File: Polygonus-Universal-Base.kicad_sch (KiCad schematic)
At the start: 5 parts, among them J4 Polygonus_Plugs, J5 Conn_02x04_Top_Bottom, U1 WBO-Single-Module

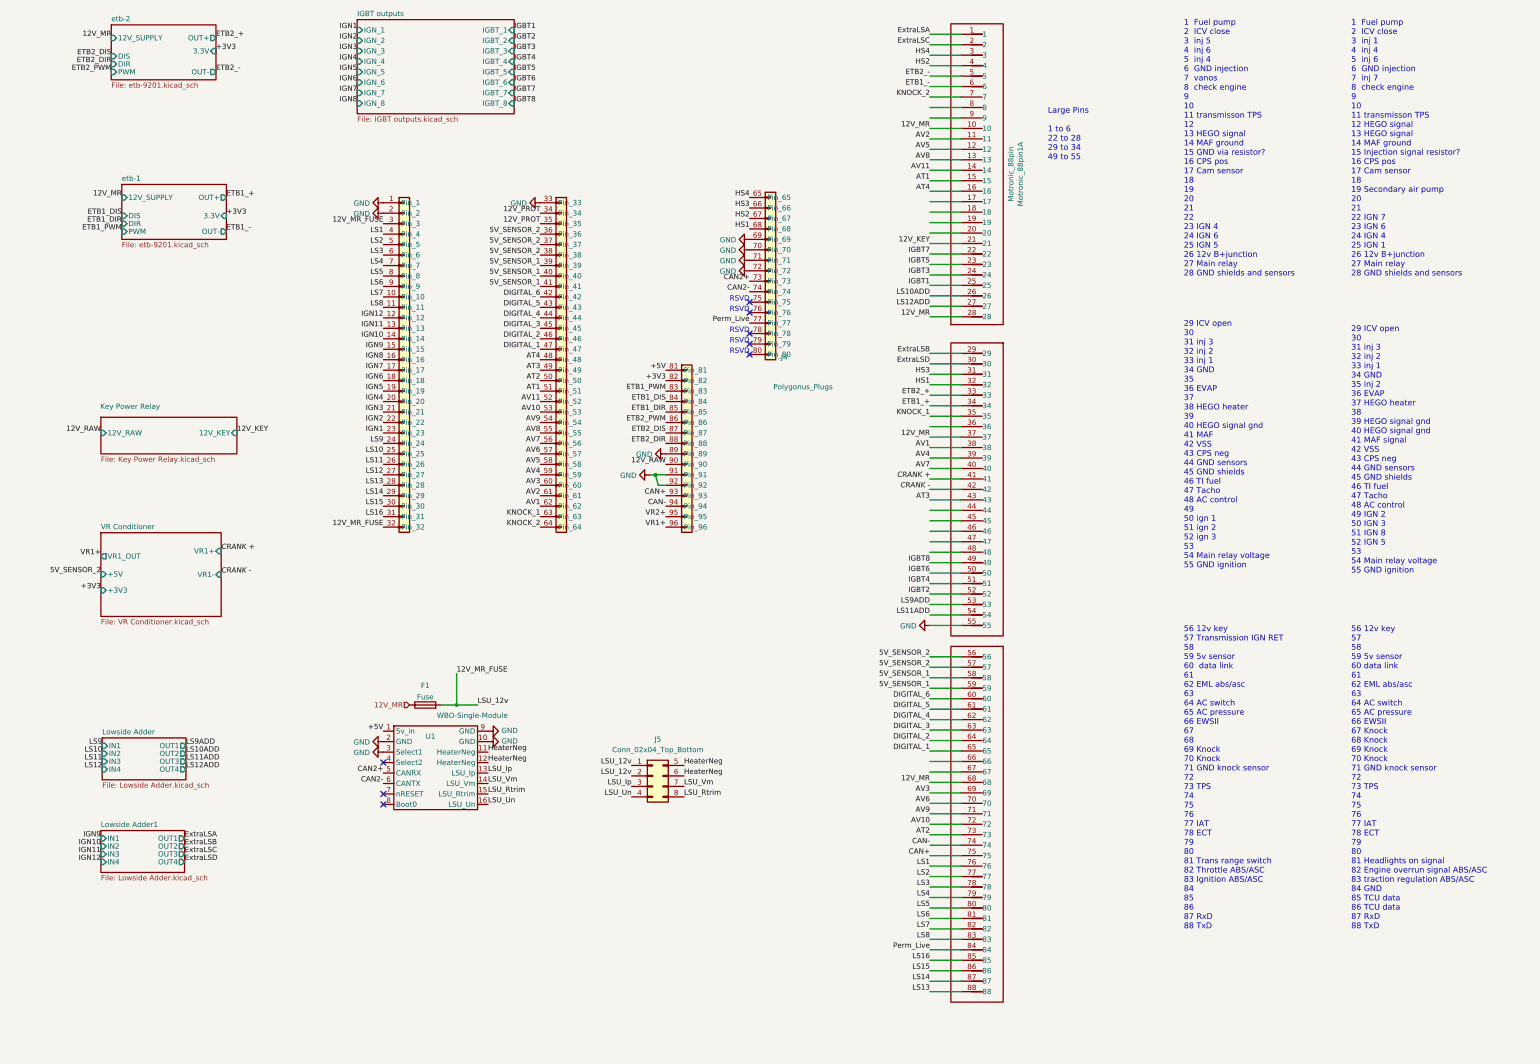
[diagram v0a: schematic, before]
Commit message: Competed board
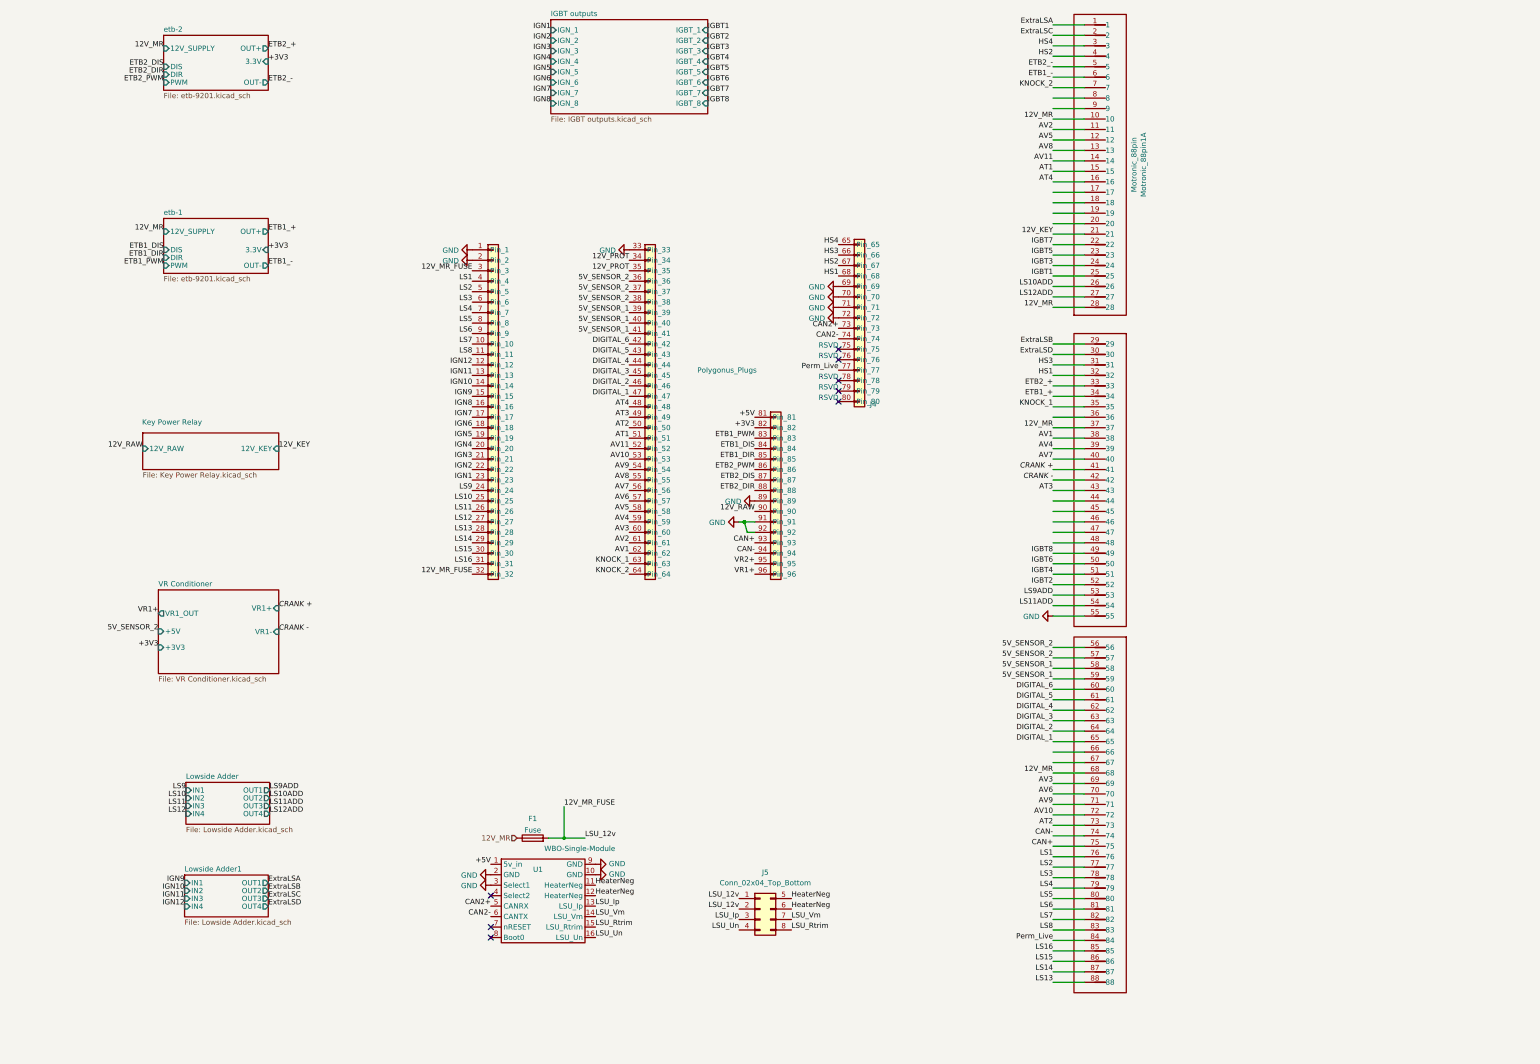
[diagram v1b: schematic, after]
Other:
- note removed: "1 Fuel pump 2 ICV close 3 inj 1 4 inj 4 5 inj 6 6 GND injection 7 inj 7 8 check engine 9 10 11 transmisson TPS 12 HEGO signal 13 HEGO signal 14 MAF ground 15 Injection signal resistor? 16 CPS pos 17 Cam sensor 18 19 Secondary air pump 20 21 22 IGN 7 23 IGN 6 24 IGN 4 25 IGN 1 26 12v B+junction 27 Main relay 28 GND shields and sensors"
- note removed: "1 Fuel pump 2 ICV close 3 inj 5 4 inj 6 5 inj 4 6 GND injection 7 vanos 8 check engine 9 10 11 transmisson TPS 12 13 HEGO signal 14 MAF ground 15 GND via resistor? 16 CPS pos 17 Cam sensor 18 19 20 21 22 23 IGN 4 24 IGN 6 25 IGN 5 26 12v B+junction 27 Main relay 28 GND shields and sensors"
- note removed: "29 ICV open 30 31 inj 3 32 inj 2 33 inj 1 34 GND 35 36 EVAP 37 38 HEGO heater 39 40 HEGO signal gnd 41 MAF 42 VSS 43 CPS neg 44 GND sensors 45 GND shields 46 TI fuel 47 Tacho 48 AC control 49 50 ign 1 51 ign 2 52 ign 3 53 54 Main relay voltage 55 GND ignition"
- note removed: "29 ICV open 30 31 inj 3 32 inj 2 33 inj 1 34 GND 35 inj 2 36 EVAP 37 HEGO heater 38 39 HEGO signal gnd 40 HEGO signal gnd 41 MAF signal 42 VSS 43 CPS neg 44 GND sensors 45 GND shields 46 TI fuel 47 Tacho 48 AC control 49 IGN 2 50 IGN 3 51 IGN 8 52 IGN 5 53 54 Main relay voltage 55 GND ignition"
- note removed: "56 12v key 57 58 59 5v sensor 60 data link 61 62 EML abs/asc 63 64 AC switch 65 AC pressure 66 EWSII 67 Knock 68 Knock 69 Knock 70 Knock 71 GND knock sensor 72 73 TPS 74 75 76 77 IAT 78 ECT 79 80 81 Headlights on signal 82 Engine overrun signal ABS/ASC 83 traction regulation ABS/ASC 84 GND 85 TCU data 86 TCU data 87 RxD 88 TxD"
- note removed: "56 12v key 57 Transmission IGN RET 58 59 5v sensor 60 data link 61 62 EML abs/asc 63 64 AC switch 65 AC pressure 66 EWSII 67 68 69 Knock 70 Knock 71 GND knock sensor 72 73 TPS 74 75 76 77 IAT 78 ECT 79 80 81 Trans range switch 82 Throttle ABS/ASC 83 Ignition ABS/ASC 84 85 86 87 RxD 88 TxD"
- note removed: "Large Pins 1 to 6 22 to 28 29 to 34 49 to 55"
- moved on the sheet: F1, J4, J5, Motronic_88pin1A, U1

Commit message: upgraded
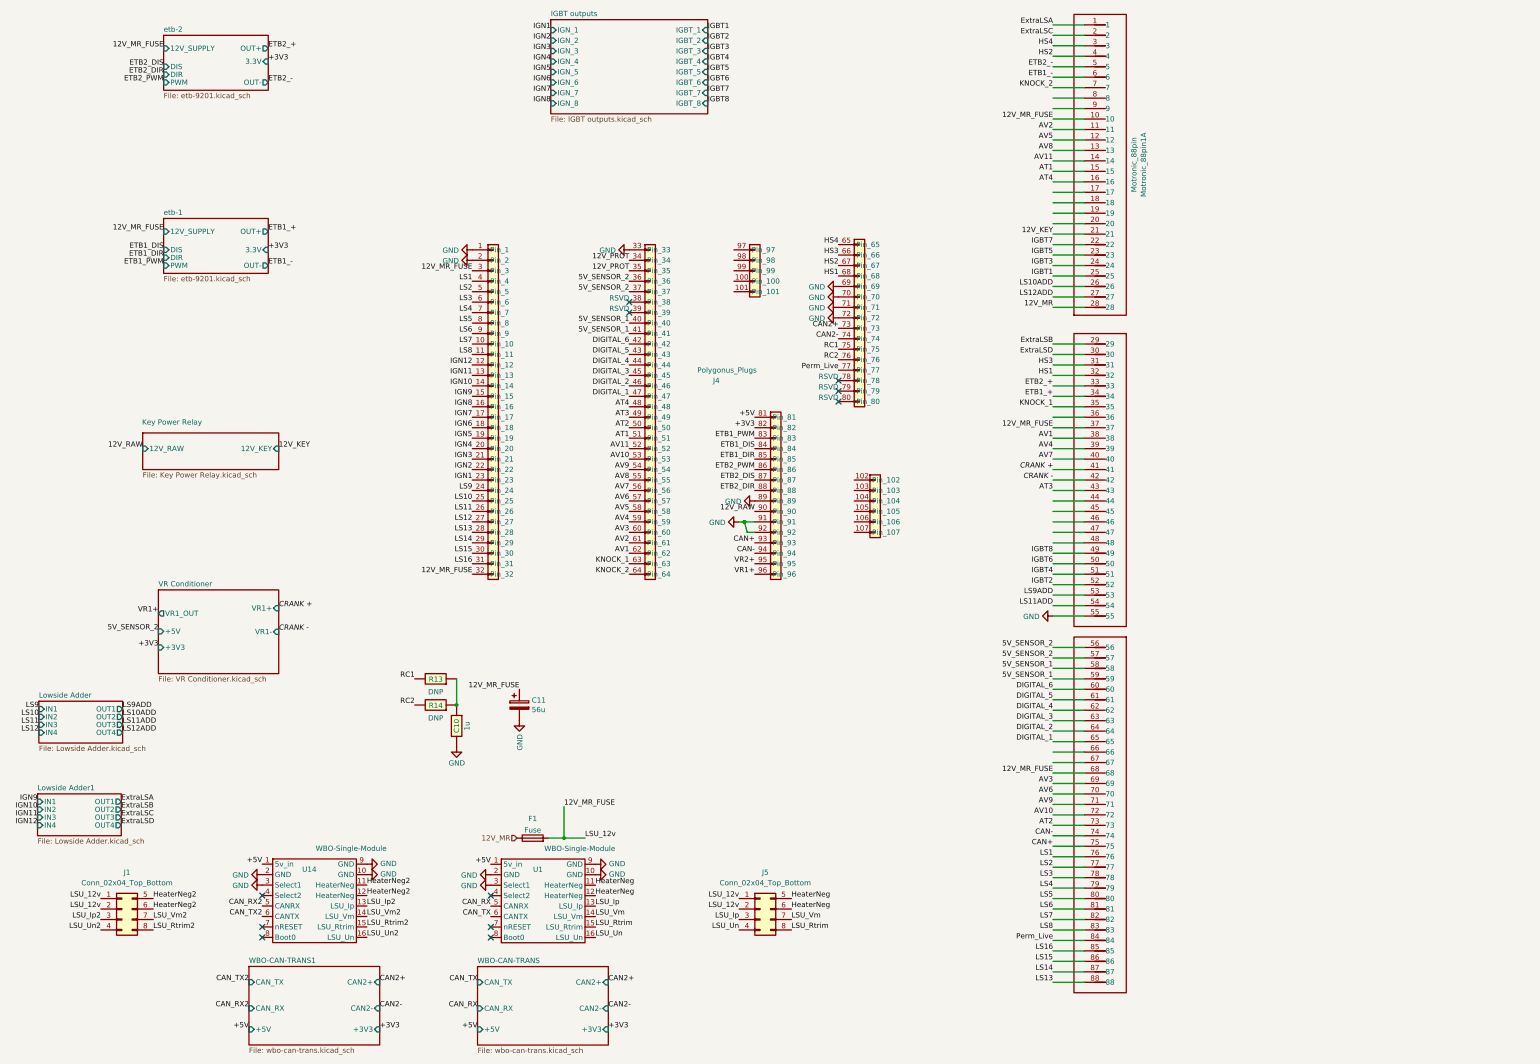
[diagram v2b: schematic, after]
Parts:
- added C10: 1u, Resistor_SMD:R_0805_2012Metric, symbol hellen-one-common:Res
- added C11: 56u, Capacitor_THT:CP_Radial_D8.0mm_P3.50mm, symbol Device:CP
- added J1: Conn_02x04_Top_Bottom, Connector_Molex:Molex_Micro-Fit_3.0_43045-0800_2x04_P3.00mm_Horizontal, symbol Connector_Generic:Conn_02x04_Top_Bottom
- added R13, R14: DNP, Resistor_SMD:R_0805_2012Metric, symbol hellen-one-common:Res
- added U14: WBO-Single-Module, wideband_module:f042_wideband_module, symbol Simon:WBO-Single-Module
- J4: footprint Simon:Polygonus-With-USB-SWD -> Simon:Polygonus_Plugs; symbol Simon:Polygonus_Plugs -> Simon:Polygonus-With-USB-SWD
- U1: footprint Simon:f042_wideband_module -> wideband_module:f042_wideband_module
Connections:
- net +5V: now also U14.1 (5v_in)
- net 12V_MR: no longer Motronic_88pin1.10, Motronic_88pin1.37, Motronic_88pin1.68
- net 12V_MR_FUSE: now also Motronic_88pin1.10, Motronic_88pin1.37, Motronic_88pin1.68, C11.1, J1.1 (Pin_1), J1.2 (Pin_2)
- net 5V_SENSOR_1: no longer J4.39 (Pin_39)
- net 5V_SENSOR_2: no longer J4.38 (Pin_38)
- net CAN2+: no longer U1.5 (CANRX)
- net CAN2-: no longer U1.6 (CANTX)
- net GND: now also C10.2, C11.2, U14.10 (GND), U14.2 (GND), U14.3 (Select1), U14.9 (GND)
- net RC1: now reaches J4.75 (Pin_75)
- net RC1: now also R13.2
- net RC2: now reaches J4.76 (Pin_76)
- net RC2: now also R14.2
- new net: C10.1, R13.1, R14.1
- new net CAN_RX: U1.5 (CANRX)
- new net CAN_RX2: U14.5 (CANRX)
- new net CAN_TX: U1.6 (CANTX)
- new net CAN_TX2: U14.6 (CANTX)
- new net HeaterNeg2: J1.5 (Pin_5), J1.6 (Pin_6), U14.11 (HeaterNeg), U14.12 (HeaterNeg)
- new net LSU_Ip2: J1.3 (Pin_3), U14.13 (LSU_Ip)
- new net LSU_Rtrim2: J1.8 (Pin_8), U14.15 (LSU_Rtrim)
- new net LSU_Un2: J1.4 (Pin_4), U14.16 (LSU_Un)
- new net LSU_Vm2: J1.7 (Pin_7), U14.14 (LSU_Vm)
- no-connect marks 8 -> 11
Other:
- added sheet WBO-CAN-TRANS (wbo-can-trans.kicad_sch)
- added sheet WBO-CAN-TRANS1 (wbo-can-trans.kicad_sch)
